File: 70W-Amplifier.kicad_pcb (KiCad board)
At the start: 2 copper layers, 170.9 x 81 mm, 35 parts, among them J1 RF_OUT, J2 RF_IN, J3 LPF_IN, J4 LPF_OUT, J5 13.8V Input, J6 PTT, K1 G5V-2, Q1 2N3906-SMD, Q2 IRF530, Q3 IRF530, T1 BN-43-202 1T:2T, T2 Ferrite 1T:3T, U1 L7805

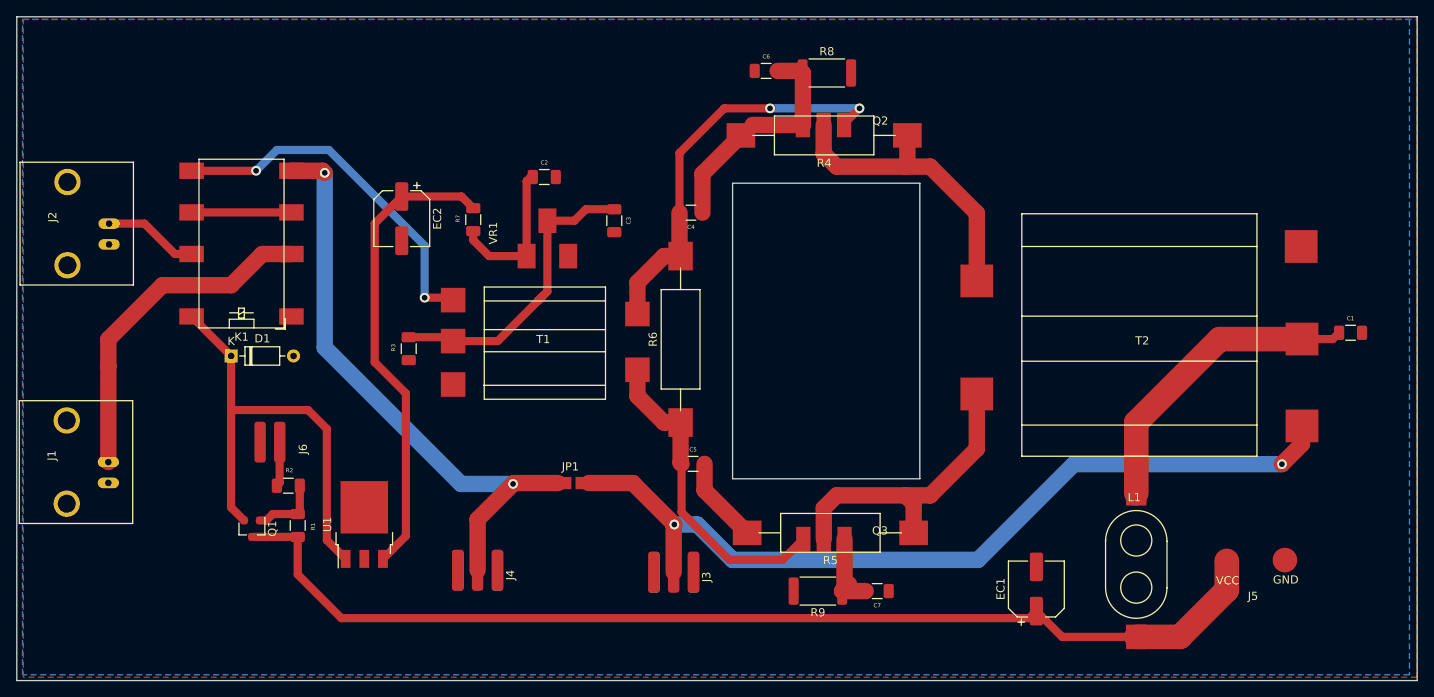
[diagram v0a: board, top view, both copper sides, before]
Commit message: CHANGED BOARD SIZE
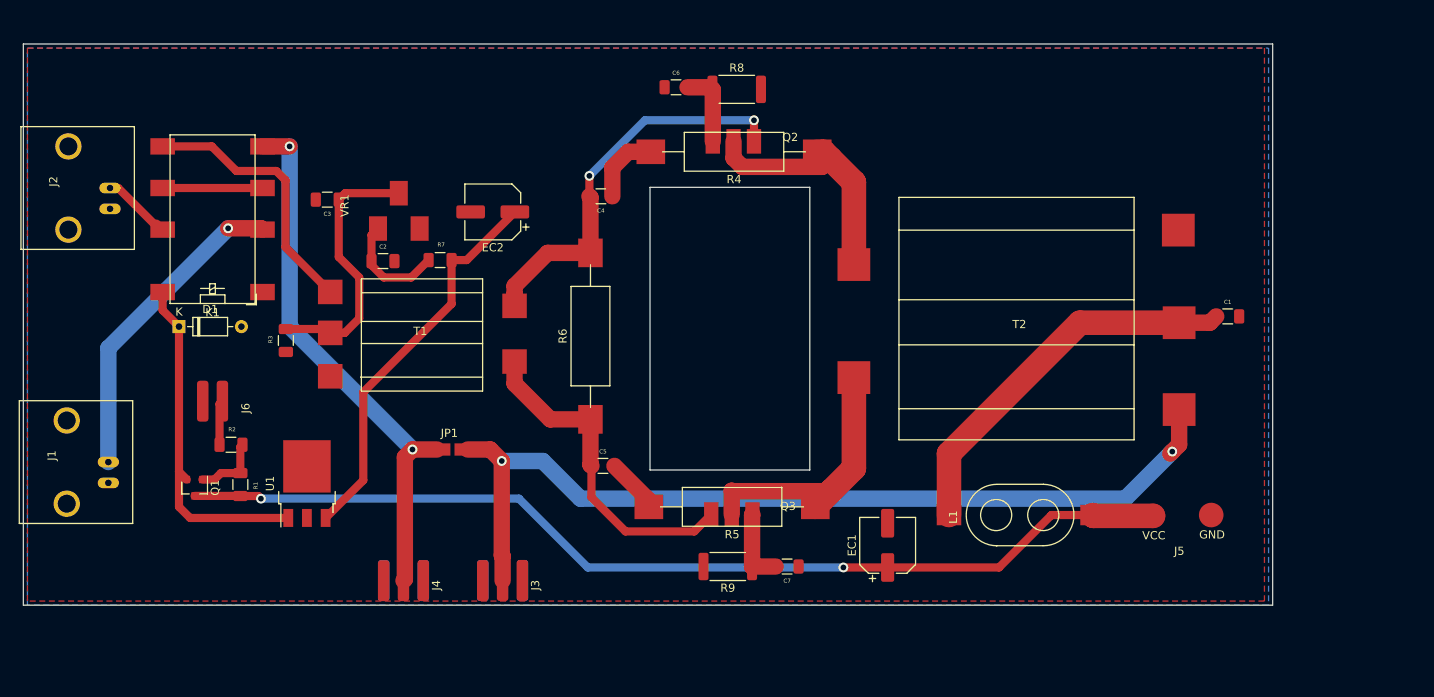
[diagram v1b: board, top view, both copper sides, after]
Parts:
- moved C3 37.3 mm to (114.1, 67.8), turned to 180 degrees
- moved C2 22.2 mm to (120.9, 70.8)
- moved J3 20.9 mm to (140.7, 112.0)
- moved EC1 18.9 mm to (182.5, 107.7)
- moved VR1 18.4 mm to (117.5, 67.0)
- moved JP1 15.3 mm to (129.5, 97.2)
- moved L1 15.2 mm to (206.5, 104.0), turned to 270 degrees
- moved C1 15.1 mm to (224.0, 77.5)
- moved T2 15.1 mm to (199.9, 97.8)
- moved R3 15.0 mm to (106.7, 82.6)
- moved T1 15.0 mm to (125.5, 69.9)
- moved R5 12.4 mm to (173.7, 103.0)
- moved Q3 11.6 mm to (163.7, 98.0)
- moved C7 11.4 mm to (170.2, 112.5)
- moved R9 11.4 mm to (163.0, 110.3)
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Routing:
- net TRANSMIT_ON: track 57.0 -> 42.3 mm
- net Net-(K1-Pad9): track 44.3 -> 32.6 mm, vias 2 -> 0
- net +12V: track 133.3 -> 123.3 mm, vias 0 -> 2
- net Net-(EC2-Pad1): track 57.7 -> 48.0 mm
- net Net-(C1-Pad1): track 38.3 -> 47.1 mm
- net LPF: track 73.3 -> 66.0 mm
- net /Q2Drain: track 37.4 -> 30.8 mm
- net Net-(J3-Pad1): track 104.9 -> 111.3 mm
- net Net-(C6-Pad2): track 15.7 -> 9.52 mm
- net Net-(C2-Pad1): track 18.5 -> 13.3 mm
- net BIAS: track 38.0 -> 33.1 mm
- net /Q3Drain: track 37.1 -> 32.8 mm
- net Net-(C5-Pad2): track 10.6 -> 6.74 mm
- net Net-(J1-PadS): track 41.7 -> 38.9 mm, vias 0 -> 1
- net Net-(C4-Pad1): track 11.1 -> 8.99 mm
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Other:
- board size 170.9 x 81 mm -> 152.5 x 68.5 mm
